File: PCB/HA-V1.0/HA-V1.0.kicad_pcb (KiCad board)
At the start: 2 copper layers, 9 parts, among them J1 Screw_Terminal_01x03, J3 Main_Relay, J4 Main_Relay, U1 ATmega328P-PU

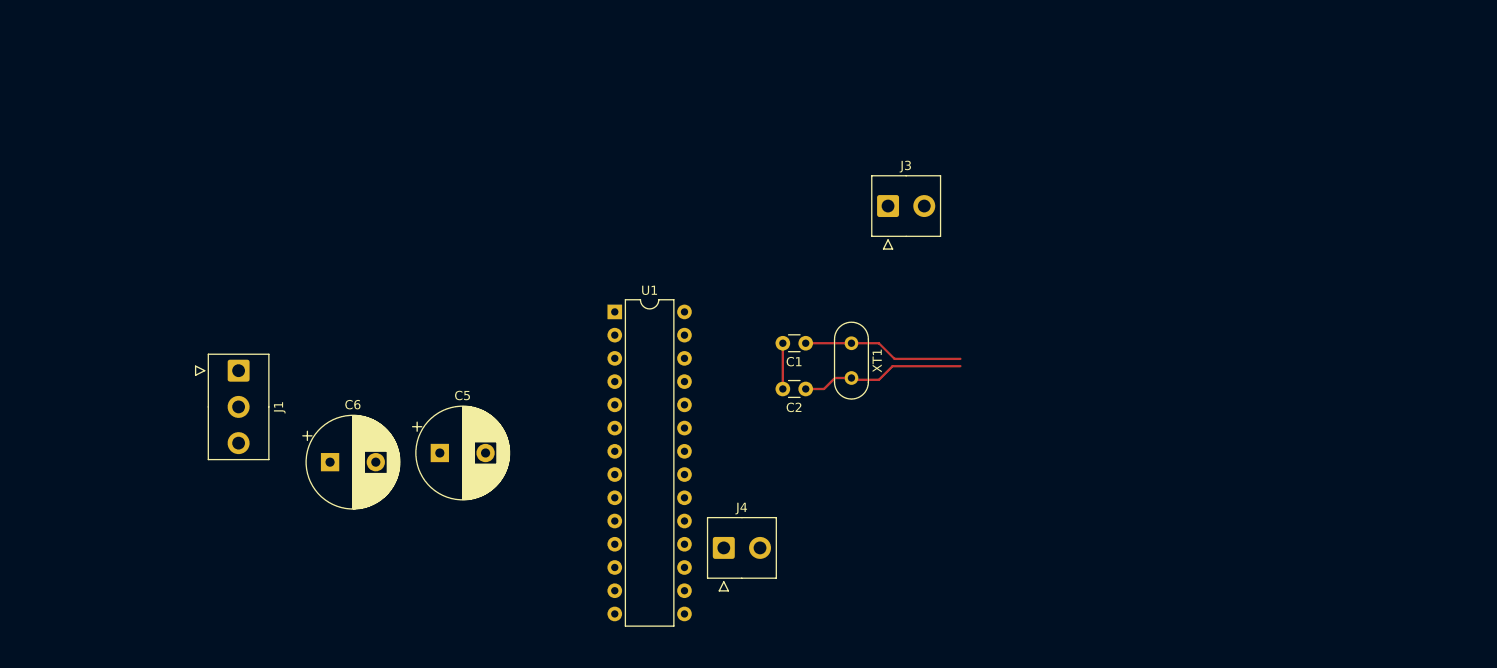
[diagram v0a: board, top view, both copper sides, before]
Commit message: Final PCB Fabrication Done
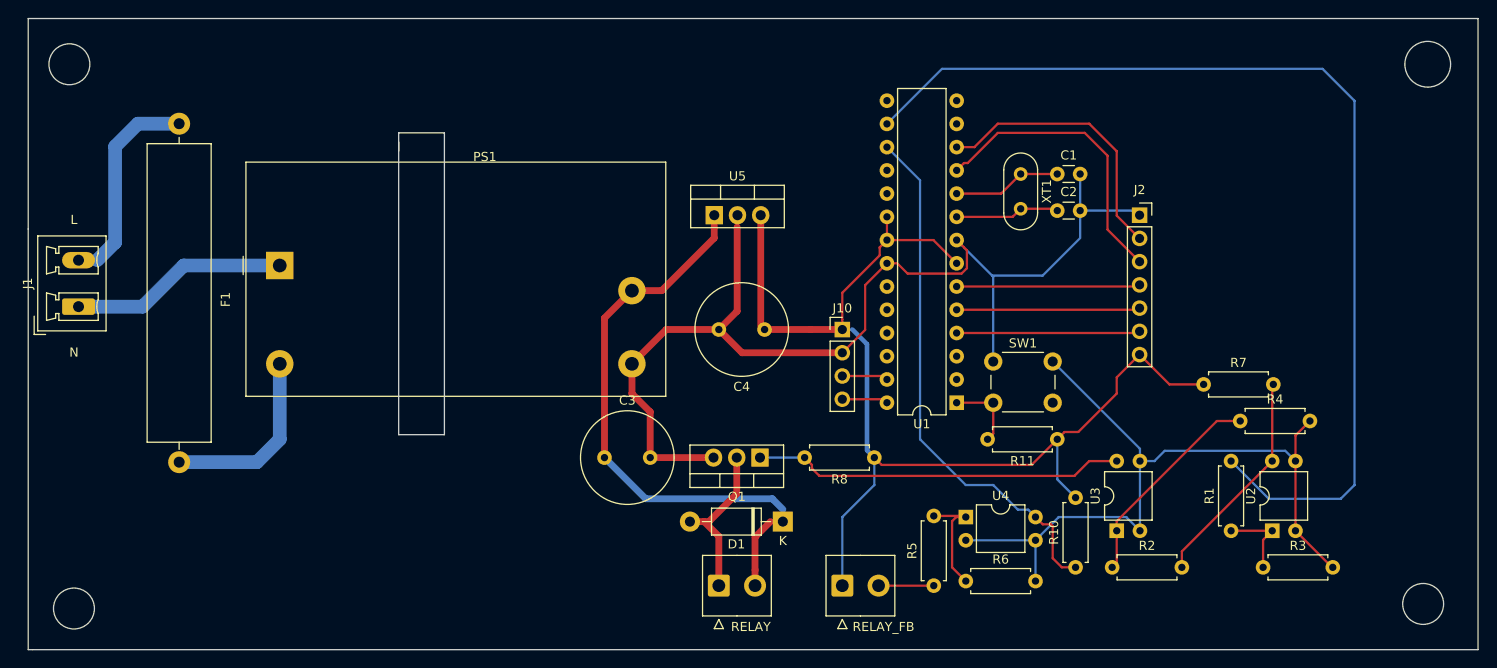
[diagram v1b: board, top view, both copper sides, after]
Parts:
- removed C5, C6: 1000uF, Capacitor_THT:CP_Radial_D10.0mm_P5.00mm
- removed J3, J4: Main_Relay, Connector_TE-Connectivity:TE_826576-2_1x02_P3.96mm_Vertical
- added C3: 1000uF, Capacitor_THT:C_Radial_D10.0mm_H16.0mm_P5.00mm, F.Cu at (113.0, 105.5)
- added C4: 1000uF, Capacitor_THT:C_Radial_D10.0mm_H16.0mm_P5.00mm, F.Cu at (130.5, 91.5)
- added D1: 1N4007, Diode_THT:D_DO-41_SOD81_P10.16mm_Horizontal, F.Cu at (132.5, 112.5)
- added F1: Main, Fuse:Fuse_SunFuse-6HP, F.Cu at (66.5, 106.0)
- added J10: I2C_LCD, Connector_PinHeader_2.54mm:PinHeader_1x04_P2.54mm_Vertical, F.Cu at (139.0, 91.5)
- added J2: BUTTON, Connector_PinSocket_2.54mm:PinSocket_1x07_P2.54mm_Vertical, F.Cu at (171.5, 79.0)
- added PS1: AC_DC, Converter_ACDC:Converter_ACDC_MeanWell_IRM-10-xx_THT, F.Cu at (77.5, 84.5)
- added Q1: IRF540N, Package_TO_SOT_THT:TO-220-3_Vertical, F.Cu at (130.0, 105.5)
- added R1: 220, Resistor_THT:R_Axial_DIN0207_L6.3mm_D2.5mm_P7.62mm_Horizontal, F.Cu at (181.5, 113.5)
- added R10: 1K, Resistor_THT:R_Axial_DIN0207_L6.3mm_D2.5mm_P7.62mm_Horizontal, F.Cu at (164.5, 117.5)
- added R11: 1K, Resistor_THT:R_Axial_DIN0207_L6.3mm_D2.5mm_P7.62mm_Horizontal, F.Cu at (162.5, 103.5)
- added R2: 220, Resistor_THT:R_Axial_DIN0207_L6.3mm_D2.5mm_P7.62mm_Horizontal, F.Cu at (168.5, 117.5)
- added R3: 1K, Resistor_THT:R_Axial_DIN0207_L6.3mm_D2.5mm_P7.62mm_Horizontal, F.Cu at (185.0, 117.5)
- added R4: 1K, Resistor_THT:R_Axial_DIN0207_L6.3mm_D2.5mm_P7.62mm_Horizontal, F.Cu at (182.5, 101.5)
- added R5: 220, Resistor_THT:R_Axial_DIN0207_L6.3mm_D2.5mm_P7.62mm_Horizontal, F.Cu at (149.0, 119.5)
- added R6: 1K, Resistor_THT:R_Axial_DIN0207_L6.3mm_D2.5mm_P7.62mm_Horizontal, F.Cu at (152.5, 119.0)
- added R7: 1K, Resistor_THT:R_Axial_DIN0207_L6.3mm_D2.5mm_P7.62mm_Horizontal, F.Cu at (178.5, 97.5)
- added R8: 1K, Resistor_THT:R_Axial_DIN0207_L6.3mm_D2.5mm_P7.62mm_Horizontal, F.Cu at (142.5, 105.5)
- added RELAY: Main_Relay, Connector_TE-Connectivity:TE_826576-2_1x02_P3.96mm_Vertical, F.Cu at (125.5, 119.5)
- added RELAY_FB: Check Relay, Connector_TE-Connectivity:TE_826576-2_1x02_P3.96mm_Vertical, F.Cu at (139.0, 119.5)
- added SW1: U1_Reset, Button_Switch_THT:SW_PUSH_6mm_H4.3mm, F.Cu at (155.5, 95.0)
- added U2: PC817, Package_DIP:DIP-4_W7.62mm, F.Cu at (186.0, 113.5)
- added U3: PC817, Package_DIP:DIP-4_W7.62mm, F.Cu at (169.0, 113.5)
- added U4: PC817, Package_DIP:DIP-4_W7.62mm, F.Cu at (152.5, 112.0)
- added U5: L7805, Package_TO_SOT_THT:TO-220-3_Vertical, F.Cu at (125.0, 79.0)
- J1: value Screw_Terminal_01x03 -> MAINS; footprint Connector_TE-Connectivity:TE_826576-3_1x03_P3.96mm_Vertical -> Connector_Phoenix_MC_HighVoltage:PhoenixContact_MCV_1,5_2-G-5.08_1x02_P5.08mm_Vertical
- moved U1 38.7 mm to (151.5, 99.5), turned to 180 degrees
- moved C2 33.7 mm to (162.5, 78.5), turned to 0 degrees
- moved C1 33.1 mm to (162.5, 74.5), turned to 0 degrees
- moved XT1 26.2 mm to (158.5, 74.5)
- moved J1 18.8 mm to (55.5, 89.0), turned to 90 degrees
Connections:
- J1 pad 1: GND -> Net-(J1-Pad1)
- J1 pad 2: 5V-P -> Net-(F1-Pad2)
- U1 pad 1: Net-(U1-Pad1) -> 328P_RESET
- U1 pad 11: Net-(U1-Pad11) -> DOWN_BTN
- U1 pad 12: Net-(U1-Pad12) -> START_BTN
- U1 pad 16: Net-(U1-Pad16) -> RL_SIGNAL
- U1 pad 17: Net-(U1-Pad17) -> RC_SCN_U1
- U1 pad 20: Net-(U1-Pad20) -> 5V-P
- U1 pad 21: Net-(U1-Pad21) -> 5V-P
- U1 pad 22: Net-(U1-Pad22) -> GND
- U1 pad 27: Net-(U1-Pad27) -> LCD_SDA
- U1 pad 28: Net-(U1-Pad28) -> LCD_SCL
- U1 pad 4: Net-(U1-Pad4) -> SET_BTN
- U1 pad 5: Net-(U1-Pad5) -> OK_BTN
- U1 pad 6: Net-(U1-Pad6) -> UP_BTN
- U1 pad 7: Net-(U1-Pad7) -> 5V-P
- U1 pad 8: Net-(U1-Pad22) -> GND
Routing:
- net GND: track 5.00 -> 205.7 mm
- net 5V-P: track 0.00 -> 127.1 mm
- net RL_SIGNAL: track 0.00 -> 112.9 mm
- net 12V-P: track 0.00 -> 65.6 mm
- net RC_SCN_U1: track 0.00 -> 58.3 mm
- net Net-(Q1-Pad1): track 0.00 -> 40.7 mm
- net DOWN_BTN: track 0.00 -> 32.3 mm
- net START_BTN: track 0.00 -> 30.4 mm
- net Net-(R2-Pad2): track 0.00 -> 24.1 mm
- net Net-(J1-Pad1): track 0.00 -> 23.9 mm
- net Net-(F1-Pad2): track 0.00 -> 23.3 mm
- net Net-(R2-Pad1): track 0.00 -> 23.3 mm
- net Net-(F1-Pad1): track 0.00 -> 20.3 mm
- net OK_BTN: track 0.00 -> 20.1 mm
- net UP_BTN: track 0.00 -> 20.1 mm
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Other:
- board outline added: 158.5 x 69 mm
- board text added: "Controller"
- board text added: "HA V1.0"
- board text added: "L"
- board text added: "N"
- board text added: "S. ROY."
